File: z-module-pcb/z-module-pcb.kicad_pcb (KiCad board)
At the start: 2 copper layers, 100.3 x 71.1 mm, 33 parts, among them K1 RELAY_VAC_VAC, K2 RELAY_VAC_EJECT, K3 REL_VAC_SENSE, P1 STEP_Z, P2 STEP_A, P3 CONTROL, P4 PWR, P5 MOT_Z, P6 MOT_A, P7 VADMI, P8 LED, P9 LIMIT_SWS, U1 4N25, U2 4N25, U3 4N25, U4 LDD300, U5 SilentStepStick, U6 SilentStepStick

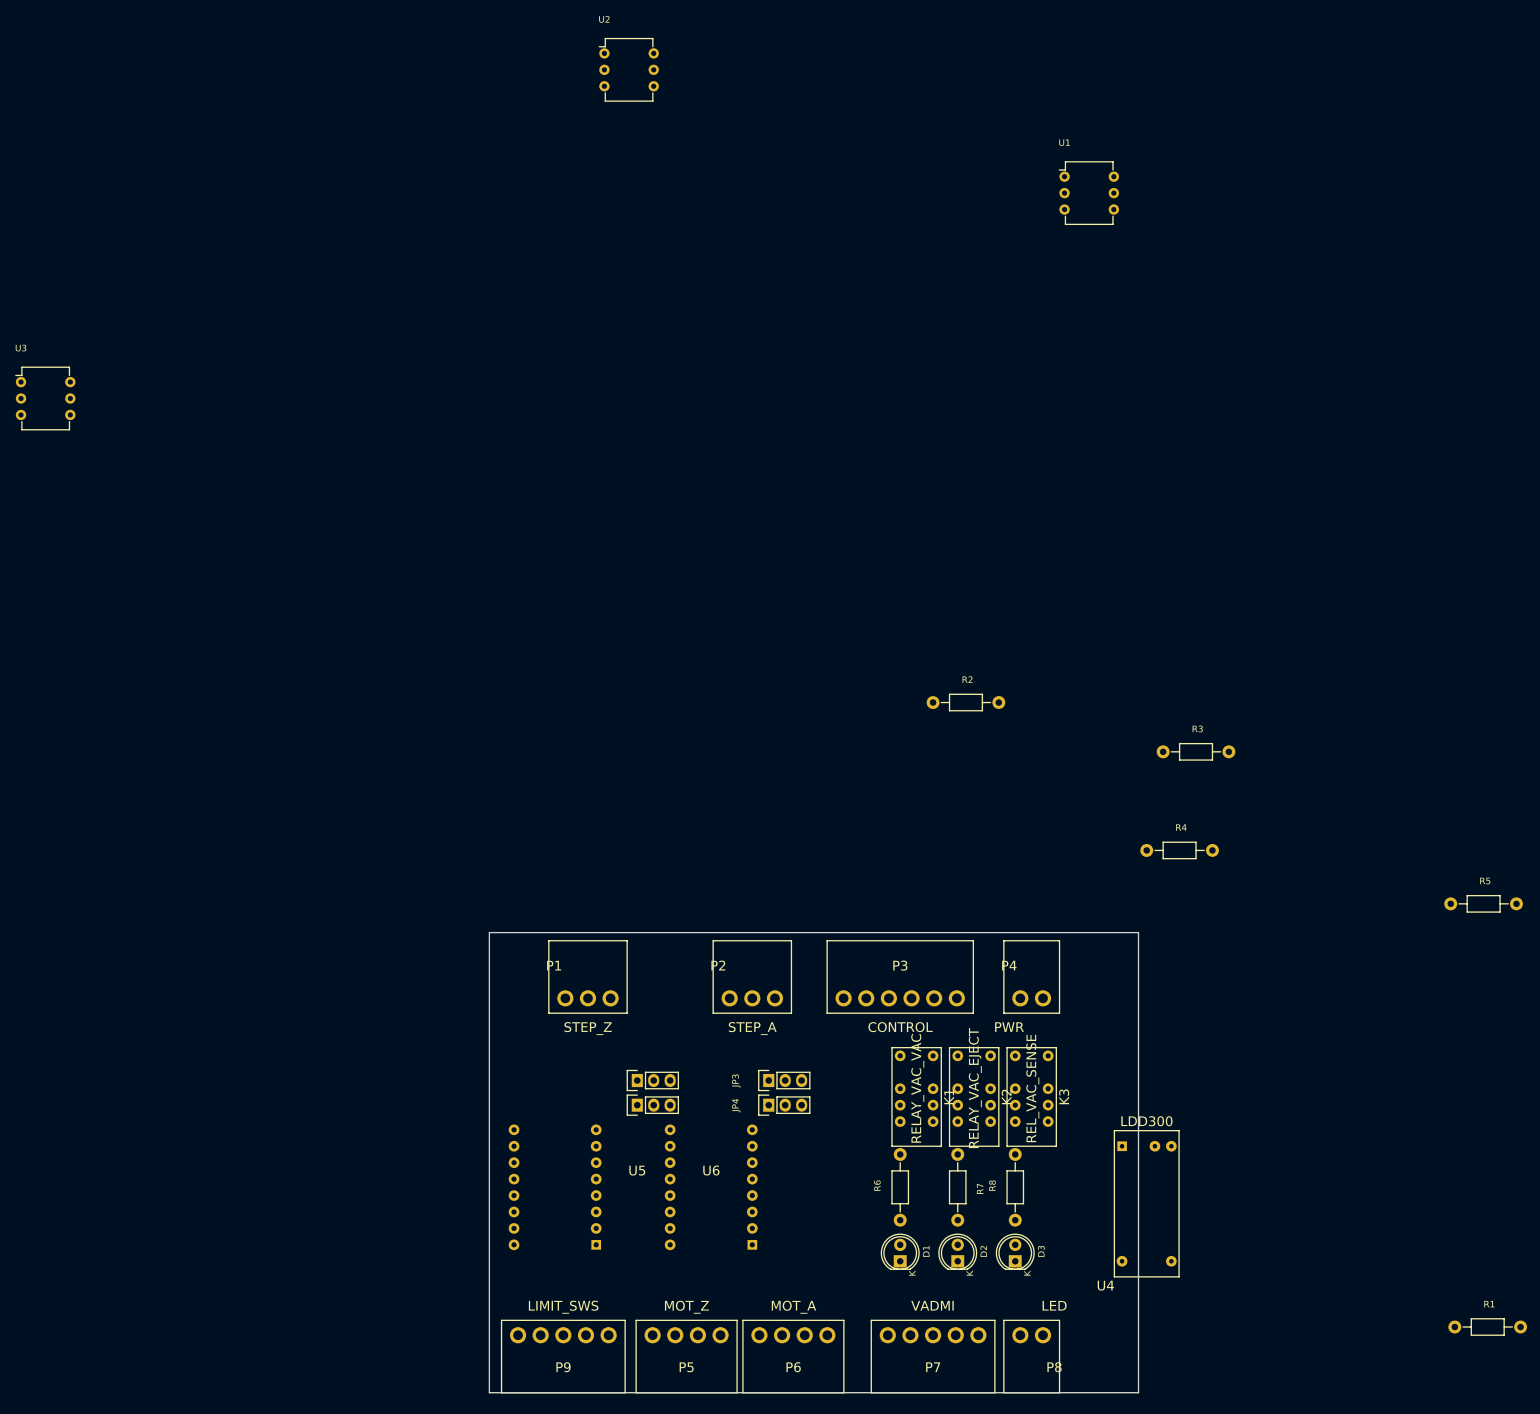
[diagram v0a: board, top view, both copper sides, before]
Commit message: Layout almost done. To be checked.
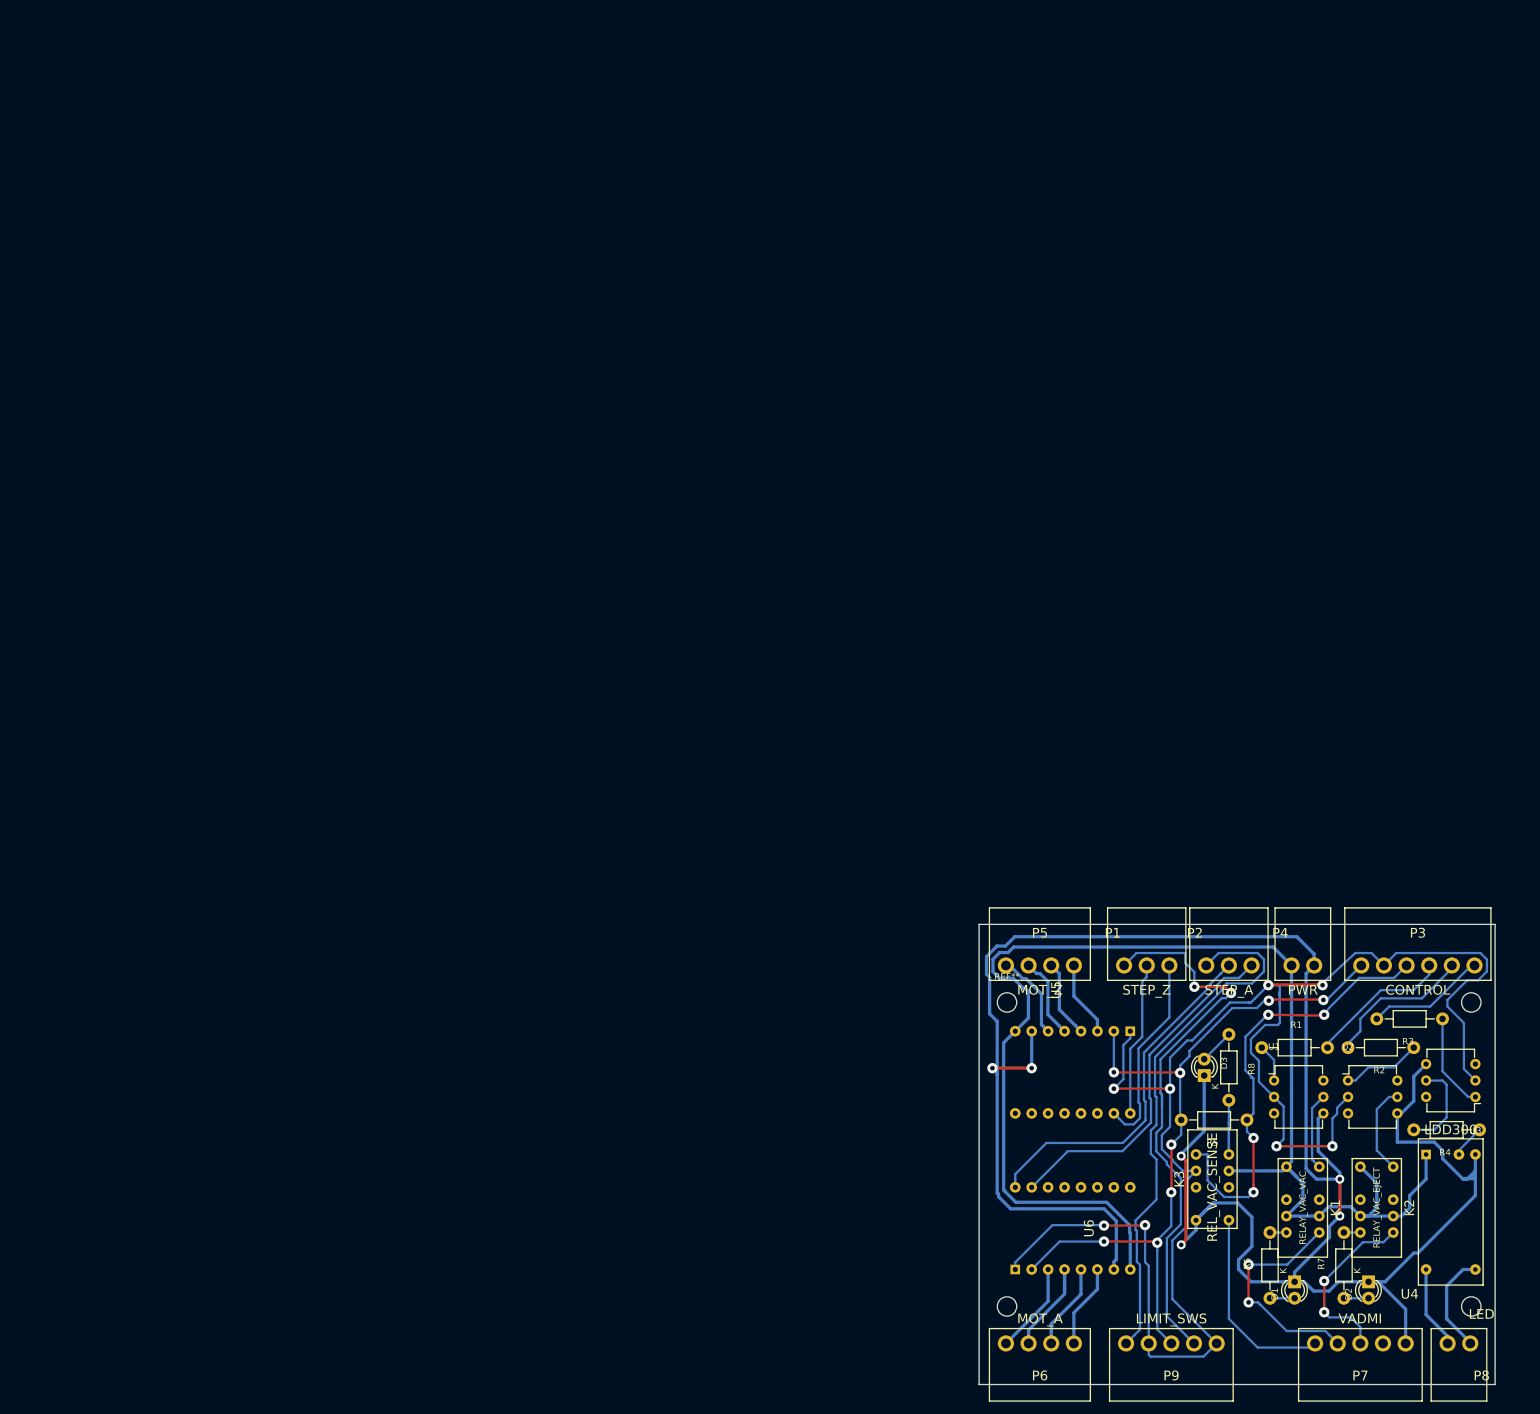
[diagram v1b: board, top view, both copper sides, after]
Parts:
- removed JP1: SZ_C2, Pin_Headers:Pin_Header_Straight_1x03
- removed JP2: SZ_C1, Pin_Headers:Pin_Header_Straight_1x03
- removed JP3: SA_C2, Pin_Headers:Pin_Header_Straight_1x03
- removed JP4: SA_C1, Pin_Headers:Pin_Header_Straight_1x03
- added REF**: MountingHole_3mm, Mounting_Holes:MountingHole_3mm, F.Cu at (78.7, 80.6)
- added REF**: MountingHole_3mm, Mounting_Holes:MountingHole_3mm, F.Cu at (78.7, 127.6)
- added REF**: MountingHole_3mm, Mounting_Holes:MountingHole_3mm, F.Cu at (150.5, 80.6)
- added REF**: MountingHole_3mm, Mounting_Holes:MountingHole_3mm, F.Cu at (150.5, 127.6)
- D1, D2, D3: footprint LEDs:LED-5MM -> LEDs:LED-3MM
- moved U3 250.5 mm to (151.1, 95.2), turned to 180 degrees
- moved U2 196.0 mm to (131.4, 92.7)
- moved U1 143.4 mm to (120.0, 92.7)
- moved P9 94.0 mm to (104.1, 133.3)
- moved U5 86.6 mm to (92.7, 91.4), turned to 270 degrees
- moved P1 86.5 mm to (100.3, 74.9)
- moved R2 83.4 mm to (136.5, 87.6), turned to 180 degrees
- moved P3 80.2 mm to (142.2, 74.9)
- moved P5 79.0 mm to (83.8, 74.9), turned to 180 degrees
- moved P2 73.8 mm to (113.0, 74.9)
- moved P8 66.1 mm to (148.6, 133.3)
- moved P7 66.1 mm to (133.3, 133.3)
- moved K2 64.5 mm to (135.9, 111.1)
- moved D2 63.6 mm to (134.6, 123.8), turned to 270 degrees
- moved K1 62.1 mm to (124.5, 111.1)
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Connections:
- net Net-(P8-Pad1) renamed /LED+
- net Net-(P8-Pad2) renamed /LED-
- P3 pad 2: VAC_SENSE -> VAC_EJECT
- P3 pad 3: VAC_EJECT -> VAC_VAC
- P3 pad 4: VAC_VAC -> VAC_SENSE
- P7 pad 1: VADMI_BN -> VADMI_BK
- P7 pad 2: VADMI_WH -> VADMI_BN
- P7 pad 3: VADMI_BK -> VADMI_WH
- P9 pad 1: STEP_Z_SW -> STEP_A_SW
- P9 pad 2: GND -> GNDD
- P9 pad 4: STEP_A_SW -> STEP_Z_SW
- P9 pad 5: GND -> GNDD
- U5 pad 10: Net-(JP2-Pad2) -> (no net)
- U5 pad 11: Net-(JP1-Pad2) -> (no net)
- U6 pad 10: Net-(JP4-Pad2) -> (no net)
- U6 pad 11: Net-(JP3-Pad2) -> (no net)
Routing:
- net GND: track 0.00 -> 355.0 mm, vias 0 -> 6
- net GNDD: track 0.00 -> 268.6 mm, vias 0 -> 8
- net +24V: track 0.00 -> 211.4 mm
- net +3V3: track 0.00 -> 119.3 mm, vias 0 -> 8
- net STEP_Z_SW: track 0.00 -> 87.7 mm, vias 0 -> 2
- net STEP_A_SW: track 0.00 -> 82.1 mm
- net VAC_SENSE: track 0.00 -> 69.5 mm, vias 0 -> 4
- net STEP_A_DIR: track 0.00 -> 55.1 mm
- net STEP_A_STP: track 0.00 -> 54.8 mm
- net VADMI_BN: track 0.00 -> 35.4 mm, vias 0 -> 2
- net STEP_Z_STP: track 0.00 -> 30.8 mm
- net VADMI_BK: track 0.00 -> 30.7 mm
- net VADMI_WH: track 0.00 -> 27.7 mm, vias 0 -> 2
- net STEP_Z_DIR: track 0.00 -> 23.9 mm
- net VAC_EJECT: track 0.00 -> 23.3 mm
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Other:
- board size 100.3 x 71.1 mm -> 79.8 x 71.1 mm
- net class BoomYa added: clearance 0.5, trace_width 0.5, via_dia 1.4, via_drill 0.7
- net class Default: clearance 0.2 -> 0.5; trace_width 0.25 -> 0.35; via_dia 0.6 -> 1.6; via_drill 0.4 -> 0.7
- rule trace_clearance: 0.2 -> 0.5
- rule trace_min: 0.2 -> 0.35
